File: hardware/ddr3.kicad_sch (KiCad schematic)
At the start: 31 parts, among them U2 H5TQ4G83EFR, U3 H5TQ4G83EFR

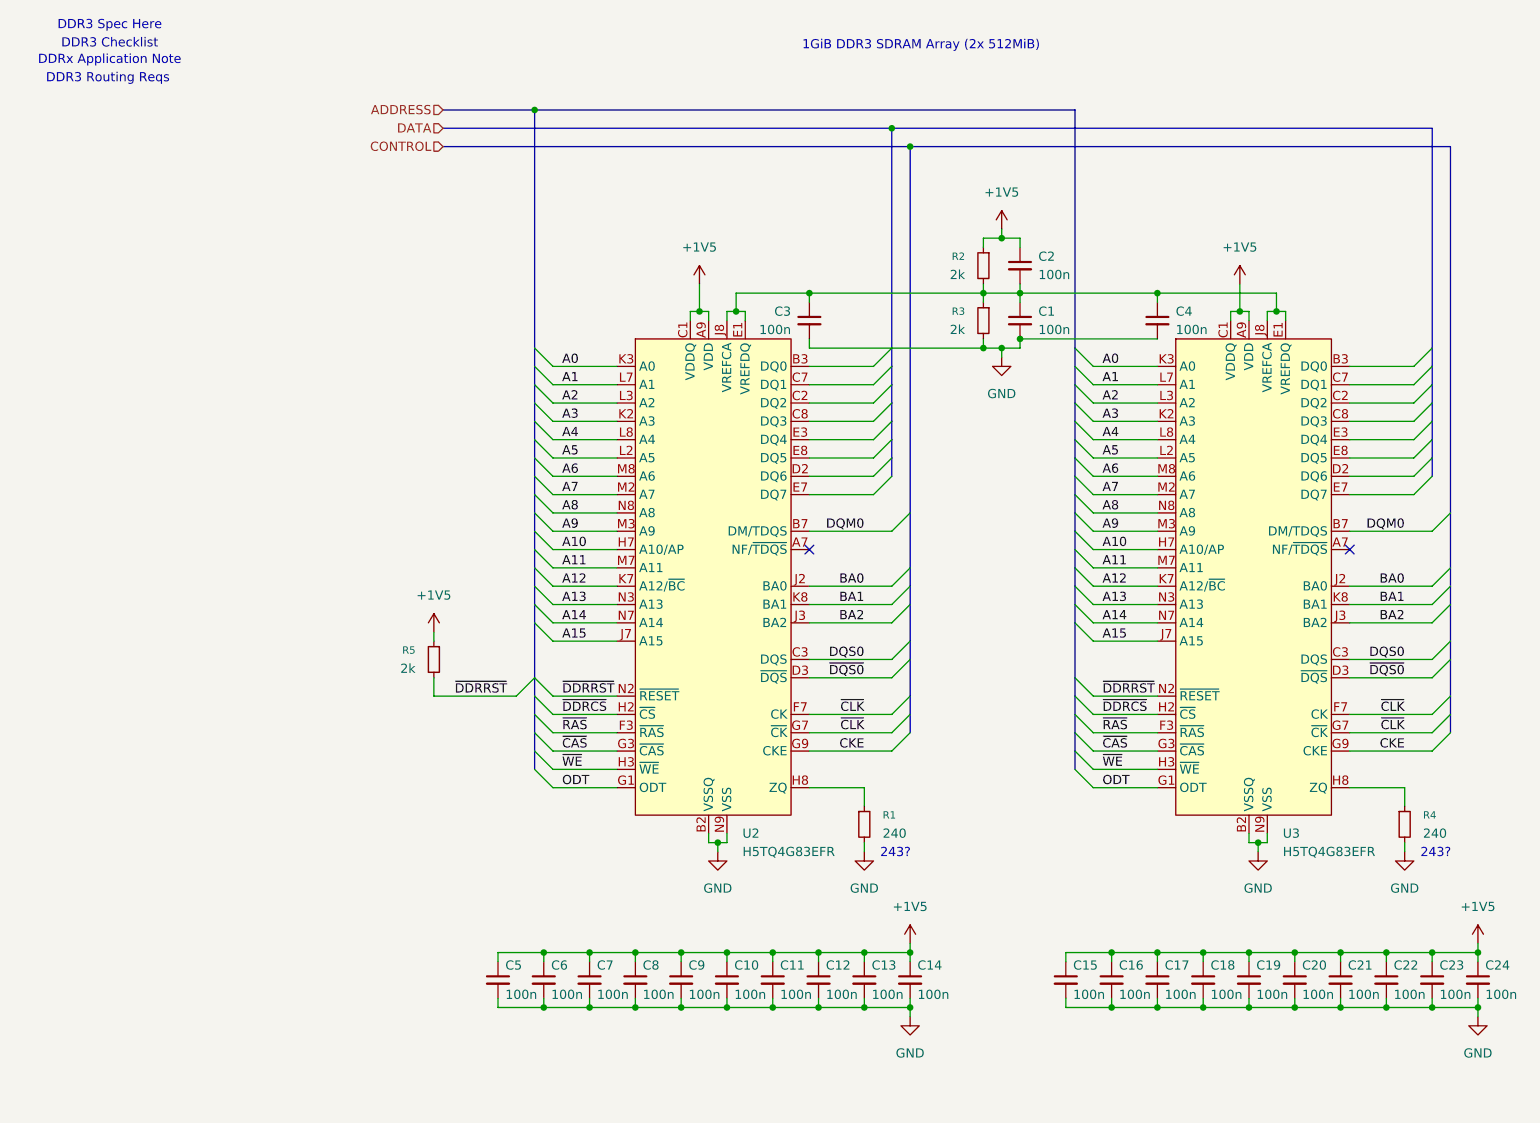
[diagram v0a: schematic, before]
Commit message: Update
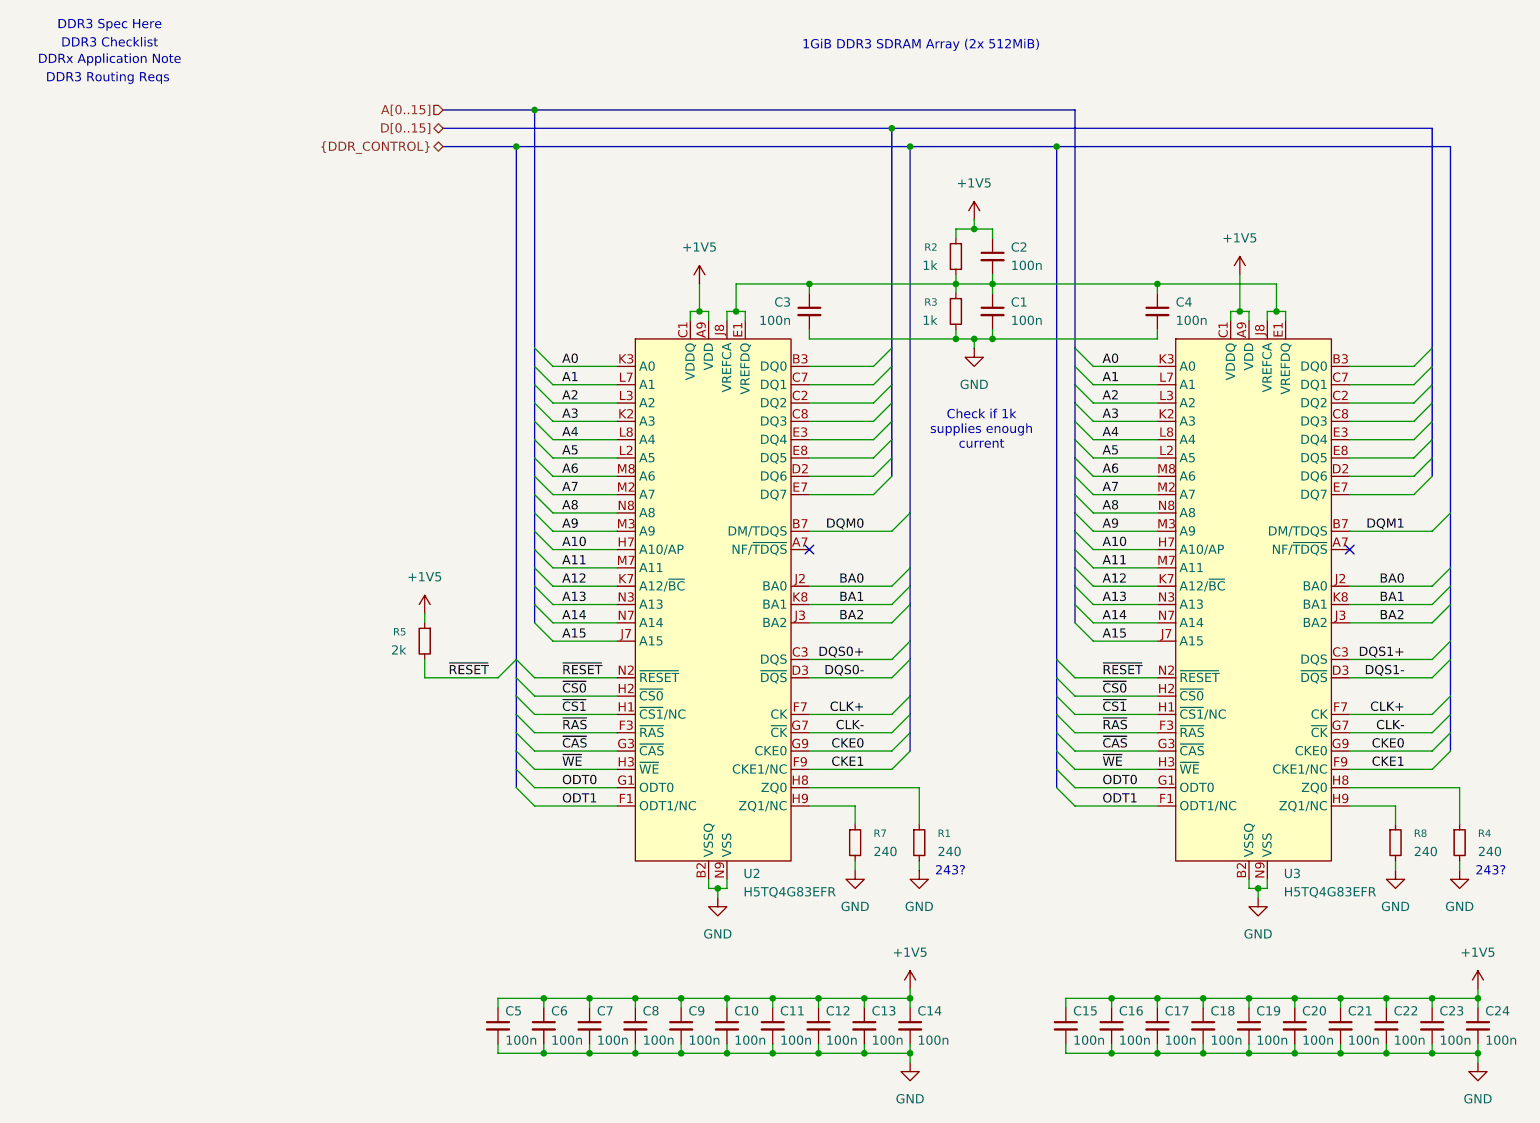
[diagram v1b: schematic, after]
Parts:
- added R7, R8: 240, Resistor_SMD:R_0201_0603Metric, symbol Device:R_Small
- R2, R3: value 2k -> 1k
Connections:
- net DQM0: no longer U3.B7 (DM/TDQS)
- net GND: now also R7.2, R8.2
- net CKE renamed CKE0
- net DQS0 renamed DQS0+
- net DQS0+: no longer U3.C3 (DQS)
- net ODT renamed ODT0
- net ~{CLK} renamed CLK+
- net CLK+: no longer U2.G7 (~{CK}), U3.G7 (~{CK})
- net ~{DDRCS} renamed ~{CS0}
- net ~{DDRRST} renamed ~{RESET}
- net ~{DQS0} renamed DQS0-
- net DQS0-: no longer U3.D3 (~{DQS})
- new net: R8.1, U3.H9 (ZQ1/NC)
- new net: R7.1, U2.H9 (ZQ1/NC)
- new net CKE1: U2.F9 (CKE1/NC), U3.F9 (CKE1/NC)
- new net CLK-: U2.G7 (~{CK}), U3.G7 (~{CK})
- new net DQM1: U3.B7 (DM/TDQS)
- new net DQS1+: U3.C3 (DQS)
- new net DQS1-: U3.D3 (~{DQS})
- new net ODT1: U2.F1 (ODT1/NC), U3.F1 (ODT1/NC)
- new net ~{CS1}: U2.H1 (~{CS1}/NC), U3.H1 (~{CS1}/NC)
- now unconnected: U2.A3 (NC), U3.A3 (NC)
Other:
- note added: "Check if 1k supplies enough current"
- moved on the sheet: C1, C10, C11, C12, C13, C14, C15, C16, C17, C18, C19, C2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
